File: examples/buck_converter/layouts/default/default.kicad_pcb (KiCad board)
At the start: 2 copper layers, 14 parts

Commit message: before claude rip
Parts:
- R4: value 162000Ω -> 95300Ω; footprint UNI_ROYAL_0402WGF1623TCE:R0402 -> Vishay_Intertech_CRCW040295K3FKED:R0402
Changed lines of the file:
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@@
 		)
 	)
-	(footprint "UNI_ROYAL_0402WGF1623TCE:R0402"
+	(footprint "Vishay_Intertech_CRCW040295K3FKED:R0402"
 		(layer "F.Cu")
 		(at 0 -10 0)
@@
 			)
 		)
-		(property "Value" "162000Ω"
+		(property "Value" "95300Ω"
 			(at 0 4)
 			(layer "F.Fab")
@@
 			)
 		)
-		(property "LCSC" "C54068"
+		(property "LCSC" "C4115778"
 			(at 0 0 0)
 			(layer "User.9")
 			(hide yes)
 		)
-		(property "Manufacturer" "UNI-ROYAL(Uniroyal Elec)"
+		(property "Manufacturer" "Vishay Intertech"
 			(at 0 0 0)
 			(layer "User.9")
@@
 			(hide yes)
 		)
-		(property "PARAM_resistance" "{\"type\": \"Quantity_Interval_Disjoint\", \"data\": {\"intervals\": {\"type\": \"Numeric_Interval_Disjoint\", \"data\": {\"intervals\": [{\"type\": \"Numeric_Interval\", \"data\": {\"min\": 160380.00003620982, \"max\": 163619.99996379018}}]}}, \"unit\": \"ohm\"}}"
+		(property "PARAM_resistance" "{\"type\": \"Quantity_Interval_Disjoint\", \"data\": {\"intervals\": {\"type\": \"Numeric_Interval_Disjoint\", \"data\": {\"intervals\": [{\"type\": \"Numeric_Interval\", \"data\": {\"min\": 94347.00002130121, \"max\": 96252.99997869879}}]}}, \"unit\": \"ohm\"}}"
 			(at 0 0 0)
 			(layer "User.9")
 			(hide yes)
 		)
-		(property "Partnumber" "0402WGF1623TCE"
+		(property "Partnumber" "CRCW040295K3FKED"
 			(at 0 0 0)
 			(layer "User.9")
 			(hide yes)
 		)
-		(property "Datasheet" "https://www.lcsc.com/datasheet/lcsc_datasheet_2206010000_UNI-ROYAL-Uniroyal-Elec-0402WGF1623TCE_C54068.pdf"
+		(property "Datasheet" "https://wmsc.lcsc.com/wmsc/upload/file/pdf/v2/lcsc/2312131014_Vishay-Intertech-CRCW040295K3FKED_C4115778.pdf"
 			(at 0 0 0)
 			(layer "User.9")
 			(hide yes)
 		)
-		(property "resistance" "162000±1.0%Ω"
+		(property "resistance" "95300±1.0%Ω"
 			(at 0 0 0)
 			(layer "User.9")
@@
 			(hide yes)
 		)
-		(property "max_voltage" "50V"
+		(property "max_voltage" "ℝ+V"
 			(at 0 0 0)
 			(layer "User.9")
@@
 			(hide yes)
 		)
-		(property "lcsc_id" "C54068"
+		(property "lcsc_id" "C4115778"
 			(at 0 0 0)
 			(layer "User.9")
@@
 		)
 		(embedded_fonts no)
-		(model "${KIPRJMOD}/../../parts/UNI_ROYAL_0402WGF1623TCE/R0402_L1.0-W0.5-H0.4.step"
+		(model "${KIPRJMOD}/../../parts/Vishay_Intertech_CRCW040295K3FKED/R0402_L1.0-W0.5-H0.4.step"
 			(offset
 				(xyz 0 0 -0)

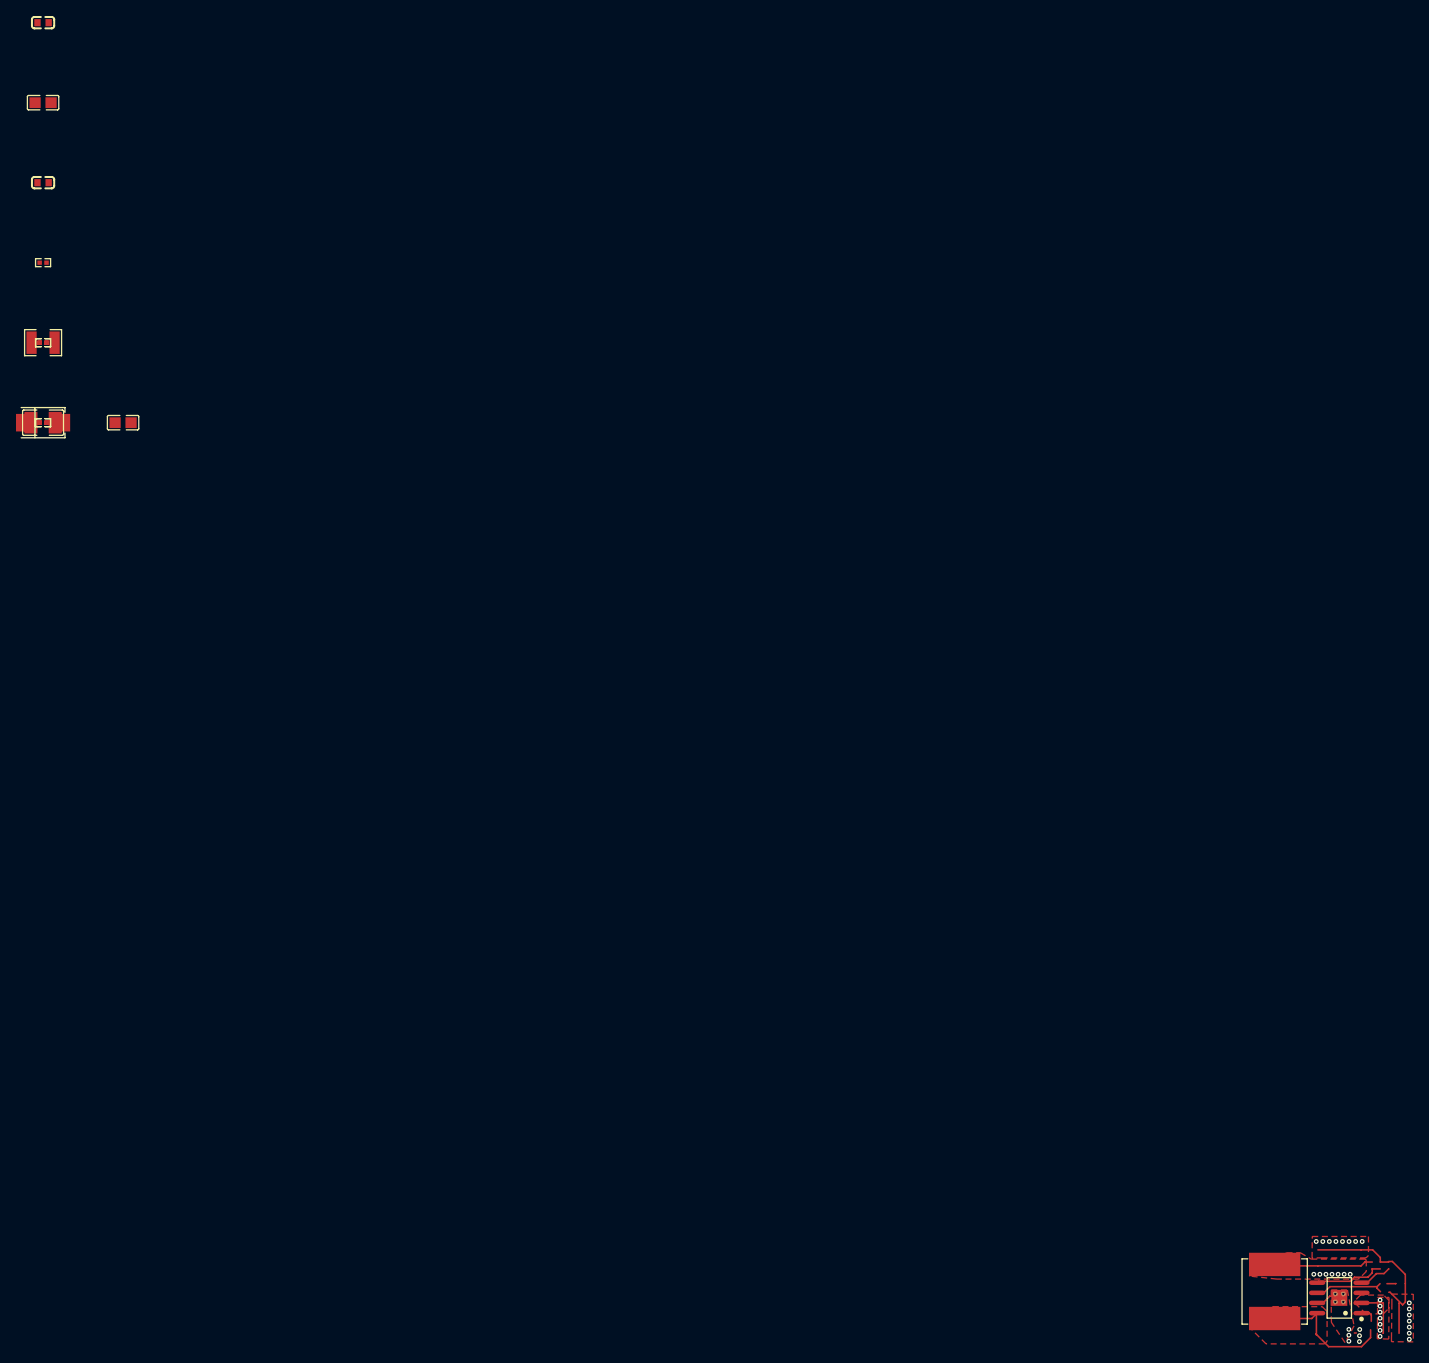
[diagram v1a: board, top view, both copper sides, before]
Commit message: checkin from server
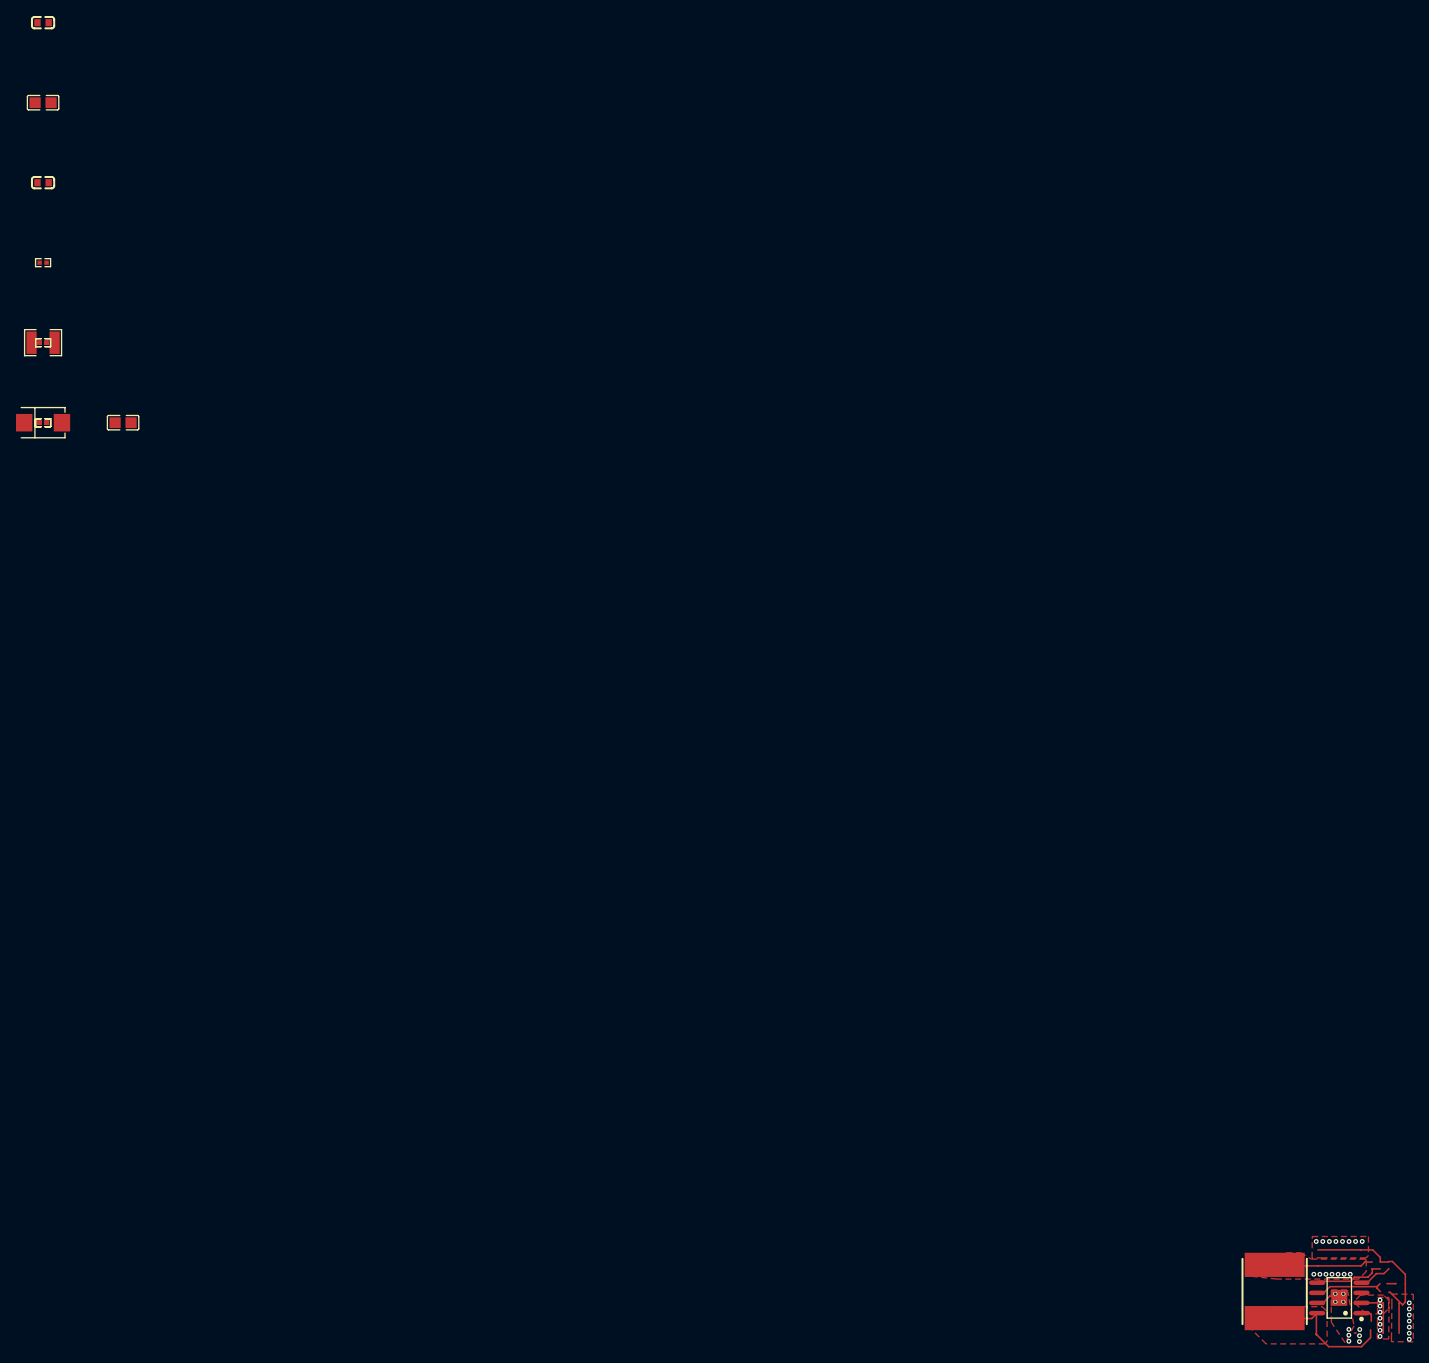
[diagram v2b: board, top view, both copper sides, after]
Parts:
- removed C5: 0F, Chinocera_HGC1210R5107M160NSVK:C1210
- added R7: 91000Ω, YAGEO_RC0402FR_0791KL:R0402, F.Cu at (0.00, 0.00)
- C3: footprint YAGEO_CC0603JRNPO9BN8R2:C0603 -> Samsung_Electro_Mechanics_CL10C470JB8NNNC:C0603
- C4: footprint FH_0805B333K500NT:C0805 -> FH_0805B472K500NT:C0805
- L1: footprint Sunlord_SWPA8040S2R2MT:IND-SMD_L8.0-W8.0_SWPA8040S -> YJYCOIN_YNR8040_6R8M:IND-SMD_L8.0-W8.0
- R1: value 7680Ω -> 10200Ω; footprint UNI_ROYAL_0402WGF7681TCE:R0402 -> UNI_ROYAL_0402WGF1022TCE:R0402
- R2: value 40200Ω -> 53600Ω; footprint UNI_ROYAL_0402WGF4022TCE:R0402 -> UNI_ROYAL_0402WGF5362TCE:R0402
- R3: value 23700Ω -> 16900Ω; footprint YAGEO_RC0402FR_0723K7L:R0402 -> UNI_ROYAL_0402WGF1692TCE:R0402
- R4: value 95300Ω -> 240000Ω; footprint Vishay_Intertech_CRCW040295K3FKED:R0402 -> FOJAN_FRC0402F2403TS:R0402
- R5: value 100000Ω -> 450000Ω; footprint UNI_ROYAL_0402WGF1003TCE:R0402 -> FOJAN_FRC0402F4503TS:R0402
- moved R1 10.0 mm to (0.00, 0.00)
- moved R2 10.0 mm to (0.00, -10.0)
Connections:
- net c_out-power-hv renamed capacitors[2]-power-hv
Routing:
- net 1: track 26.8 -> 0.00 mm, vias 21 -> 0
- net EN: track 2.06 -> 26.8 mm, vias 0 -> 21
- net 0: track 0.00 -> 23.5 mm, vias 0 -> 7
- net capacitors[2]-power-hv: track 12.4 -> 0.00 mm, vias 7 -> 0
- net FB: track 9.00 -> 0.00 mm
- removed copper zone on F.Cu, net output_caps[3]-power-hv

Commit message: trying to fix interactive requirements
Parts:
- R6: value 1Ω -> 1000Ω; footprint UNI_ROYAL_1210W2F100KT5E:R1210 -> UNI_ROYAL_1210W2J0102T5E:R1210
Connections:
- net capacitors[2]-power-hv renamed capacitors[3]-power-hv
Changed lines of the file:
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@@
 	(net 2 "c_in-power-hv")
 	(net 1 "EN")
-	(net 3 "capacitors[2]-power-hv")
+	(net 3 "capacitors[3]-power-hv")
 	(net 6 "FB")
 	(footprint "Texas_Instruments_TPS54560DDAR:SOIC-8_L5.0-W4.0-P1.27-LS6.0-BL-EP2.0"
@@
 			(size 3.02 7.5)
 			(layers "F.Cu" "F.Paste" "F.Mask")
-			(net 3 "capacitors[2]-power-hv")
+			(net 3 "capacitors[3]-power-hv")
 		)
 		(embedded_fonts no)
@@
 		)
 	)
-	(footprint "UNI_ROYAL_1210W2F100KT5E:R1210"
+	(footprint "UNI_ROYAL_1210W2J0102T5E:R1210"
 		(layer "F.Cu")
 		(at 0 -10 0)
@@
 			)
 		)
-		(property "Value" "1Ω"
+		(property "Value" "1000Ω"
 			(at 0 4)
 			(layer "F.Fab")
@@
 			)
 		)
-		(property "LCSC" "C78022"
+		(property "LCSC" "C270888"
 			(at 0 0 0)
 			(layer "User.9")
@@
 			(hide yes)
 		)
-		(property "PARAM_resistance" "{\"type\": \"Quantity_Interval_Disjoint\", \"data\": {\"intervals\": {\"type\": \"Numeric_Interval_Disjoint\", \"data\": {\"intervals\": [{\"type\": \"Numeric_Interval\", \"data\": {\"min\": 0.9900000002235174, \"max\": 1.0099999997764826}}]}}, \"unit\": \"ohm\"}}"
+		(property "PARAM_resistance" "{\"type\": \"Quantity_Interval_Disjoint\", \"data\": {\"intervals\": {\"type\": \"Numeric_Interval_Disjoint\", \"data\": {\"intervals\": [{\"type\": \"Numeric_Interval\", \"data\": {\"min\": 949.9999992549419, \"max\": 1050.000000745058}}]}}, \"unit\": \"ohm\"}}"
 			(at 0 0 0)
 			(layer "User.9")
 			(hide yes)
 		)
-		(property "Partnumber" "1210W2F100KT5E"
+		(property "Partnumber" "1210W2J0102T5E"
 			(at 0 0 0)
 			(layer "User.9")
 			(hide yes)
 		)
-		(property "Datasheet" "https://www.lcsc.com/datasheet/lcsc_datasheet_2205312316_UNI-ROYAL-Uniroyal-Elec-1210W2F100KT5E_C78022.pdf"
+		(property "Datasheet" "https://www.lcsc.com/datasheet/lcsc_datasheet_2205312300_UNI-ROYAL-Uniroyal-Elec-1210W2J0102T5E_C270888.pdf"
 			(at 0 0 0)
 			(layer "User.9")
 			(hide yes)
 		)
-		(property "resistance" "1±1.0%Ω"
+		(property "resistance" "1000±5.0%Ω"
 			(at 0 0 0)
 			(layer "User.9")
@@
 			(hide yes)
 		)
-		(property "lcsc_id" "C78022"
+		(property "lcsc_id" "C270888"
 			(at 0 0 0)
 			(layer "User.9")
@@
 			(size 1.28 2.81)
 			(layers "F.Cu" "F.Paste" "F.Mask")
-			(net 3 "capacitors[2]-power-hv")
+			(net 3 "capacitors[3]-power-hv")
 		)
 		(embedded_fonts no)
-		(model "${KIPRJMOD}/../../parts/UNI_ROYAL_1210W2F100KT5E/R1210_L3.2-W2.6-H0.6.step"
+		(model "${KIPRJMOD}/../../parts/UNI_ROYAL_1210W2J0102T5E/R1210_L3.2-W2.6-H0.6.step"
 			(offset
 				(xyz 0 0 -0)
@@
 			(size 0.57 0.54)
 			(layers "F.Cu" "F.Paste" "F.Mask")
-			(net 3 "capacitors[2]-power-hv")
+			(net 3 "capacitors[3]-power-hv")
 		)
 		(embedded_fonts no)
